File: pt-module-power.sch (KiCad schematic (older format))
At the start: 30 parts, among them U1 MCP16331, U2 MCP16331, U3 MCP16331

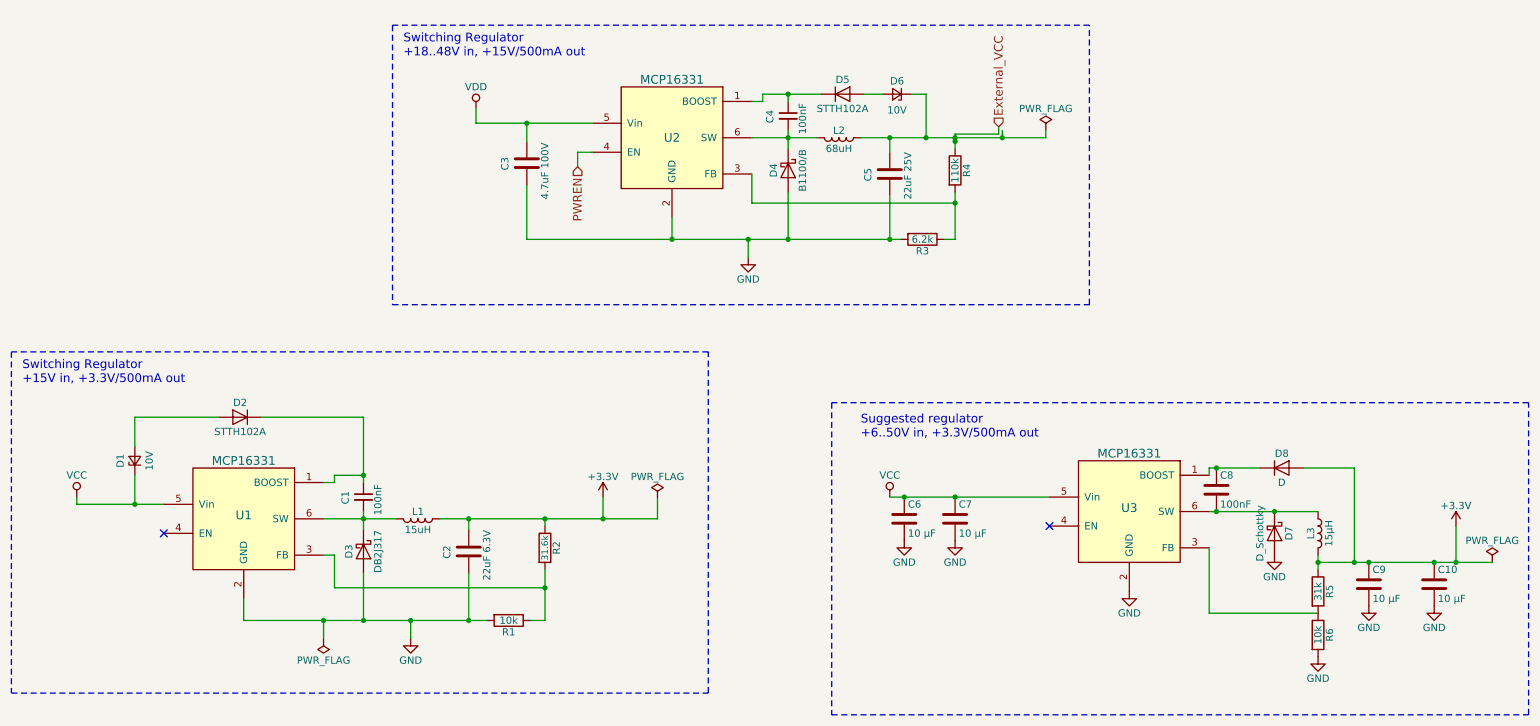
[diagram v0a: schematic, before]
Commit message: fix power scheme
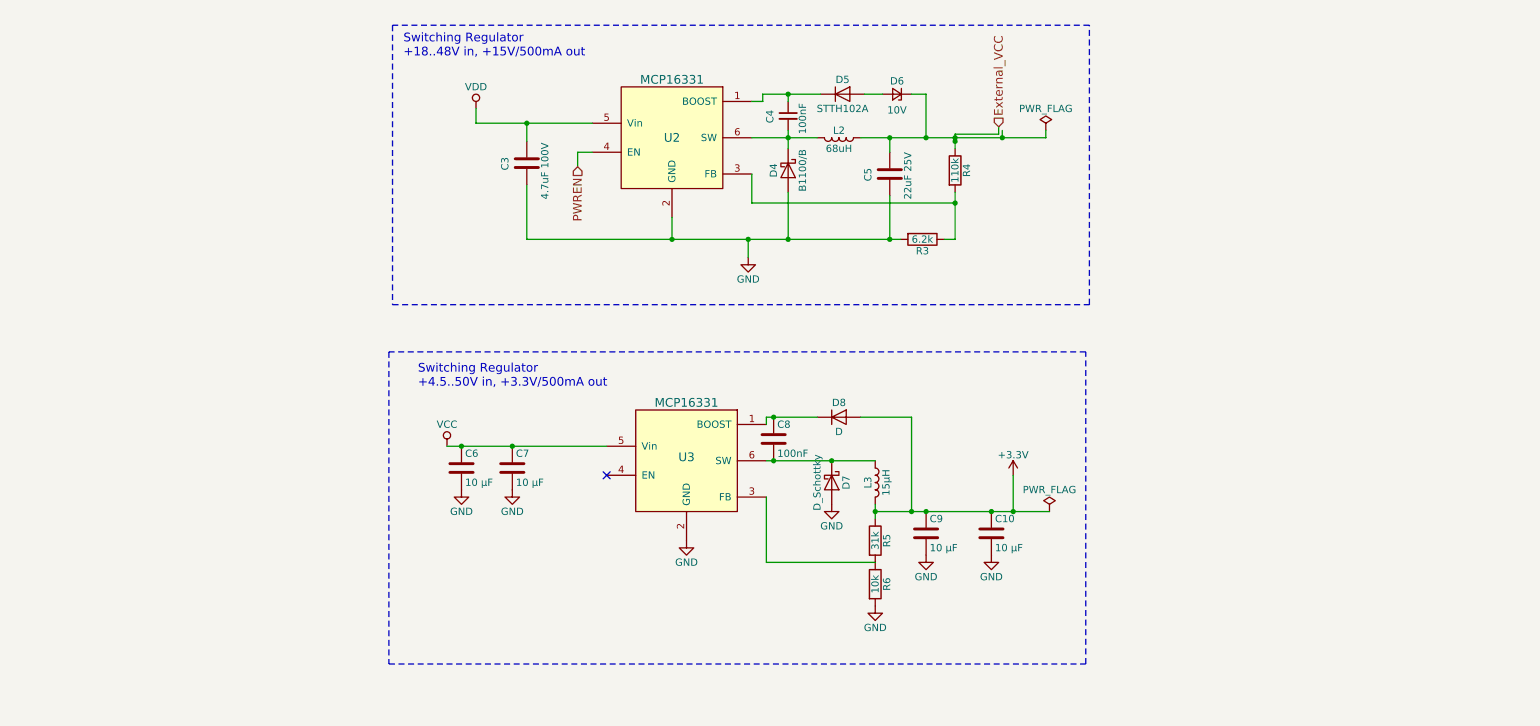
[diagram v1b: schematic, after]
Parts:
- removed C1: 100nF, symbol C_Small
- removed C2: 22uF 6.3V, symbol C
- removed D1: 10V, Diodes_SMD:D_SOD-323, symbol D_Zener_Small
- removed D2: STTH102A, Diodes_SMD:D_SMA, symbol D
- removed D3: DB2J317, Diodes_SMD:D_SOD-323, symbol D_Schottky
- removed L1: 15uH, Inductors_SMD:L_Taiyo-Yuden_NR-40xx_HandSoldering, symbol L
- removed R1: 10k, symbol R
- removed R2: 31.6k, symbol R
- removed U1: MCP16331, TO_SOT_Packages_SMD:SOT-23-6, symbol MCP16331
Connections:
- no-connect marks 2 -> 1
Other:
- note added: "Switching Regulator\n+4.5..50V in, +3.3V/500mA out"
- note removed: "Suggested regulator\n+6..50V in, +3.3V/500mA out"
- note removed: "Switching Regulator\n+15V in, +3.3V/500mA out"
- moved on the sheet: C10, C6, C7, C8, C9, D7, D8, L3, R5, R6, U3
